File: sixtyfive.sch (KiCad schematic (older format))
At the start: 204 parts, among them J1 Conn_01x12, J2 Conn_ARM_JTAG_SWD_10, Q1 BSS138, SW1 SW_Push, U1 USBLC6-2SC6, U2 STM32F072C8Tx, U3 MCP1700-3302E_SOT23

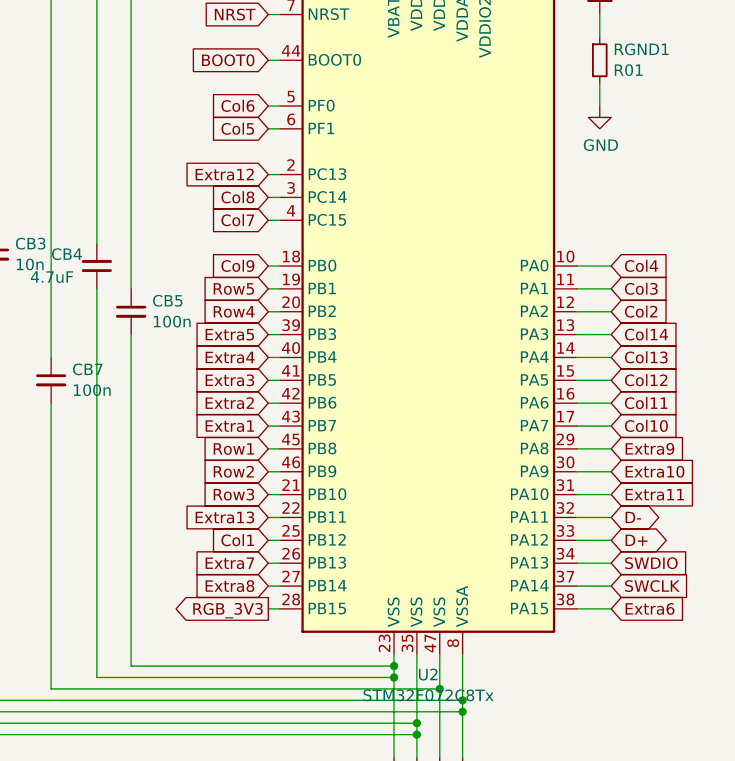
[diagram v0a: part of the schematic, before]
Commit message: Placed... everything? wired everything?
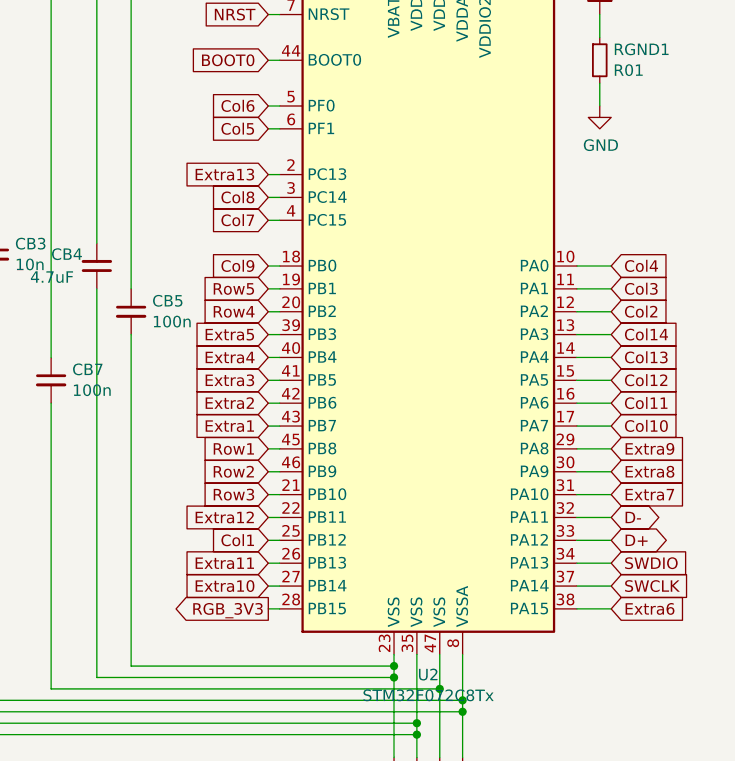
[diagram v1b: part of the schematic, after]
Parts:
- J2: footprint (none) -> sixtyfive:Conn_ARM_JTAG_SWD_10
- SW1: footprint (none) -> sixtyfive:smdPushBtn
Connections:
- net Extra10: now also U2.27 (PB14); no longer U2.30 (PA9)
- net Extra11: now also U2.26 (PB13); no longer U2.31 (PA10)
- net Extra12: now also U2.22 (PB11); no longer U2.2 (PC13)
- net Extra13: now also U2.2 (PC13); no longer U2.22 (PB11)
- net Extra7: now also U2.31 (PA10); no longer U2.26 (PB13)
- net Extra8: now also U2.30 (PA9); no longer U2.27 (PB14)
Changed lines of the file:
@@
 F 0 "J2" H 21557 20896 50  0000 R CNN
 F 1 "Conn_ARM_JTAG_SWD_10" H 21557 20805 50  0000 R CNN
-F 2 "" H 22000 20850 50  0001 C CNN
+F 2 "sixtyfive:Conn_ARM_JTAG_SWD_10" H 22000 20850 50  0001 C CNN
 F 3 "http://infocenter.arm.com/help/topic/com.arm.doc.ddi0314h/DDI0314H_coresight_components_trm.pdf" V 21650 19600 50  0001 C CNN
 	1    22000 20850
@@
 Col8
 Text GLabel 28150 16900 0    50   Input ~ 0
-Extra12
+Extra13
 Text GLabel 28150 16700 0    50   Input ~ 0
 Col5
@@
 Row1
 Text GLabel 28150 18400 0    50   Input ~ 0
-Extra13
+Extra12
 Text GLabel 28150 18300 0    50   Input ~ 0
 Row3
 Text GLabel 28150 18600 0    50   Input ~ 0
-Extra7
+Extra11
 Text GLabel 28150 18500 0    50   Input ~ 0
 Col1
@@
 RGB_3V3
 Text GLabel 28150 18700 0    50   Input ~ 0
-Extra8
+Extra10
 Wire Wire Line
 	28150 18800 28200 18800
@@
 Col11
 Text GLabel 29650 18200 2    50   Input ~ 0
-Extra10
+Extra8
 Text GLabel 29650 18100 2    50   Input ~ 0
 Extra9
 Text GLabel 29650 18300 2    50   Input ~ 0
-Extra11
+Extra7
 Text GLabel 29650 18800 2    50   Input ~ 0
 Extra6
@@
 F 0 "SW1" V 20346 19202 50  0000 R CNN
 F 1 "SW_Push" V 20255 19202 50  0000 R CNN
-F 2 "" H 20300 19450 50  0001 C CNN
+F 2 "sixtyfive:smdPushBtn" H 20300 19450 50  0001 C CNN
 F 3 "~" H 20300 19450 50  0001 C CNN
 	1    20300 19250
